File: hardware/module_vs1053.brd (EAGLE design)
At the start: 109.9 x 68.6 mm, 118 parts, among them IC1 IC_USBLC6-2, IC2 LM1117IMPX-3.3, IC3 PIC32MX795F512, IC4 DP83848, IC5 LM1117MPX-2.5, J1 AUDIO_JACK_TRRSSMD_RA, U1 USD-SOCKETUSD, U3 VS1053-L, X2 CRYSTALS-NOGND-CFPX-217, X3 KUSBVX, Y3 CRYSTAL-GROUNDEDSMD-5X3.2

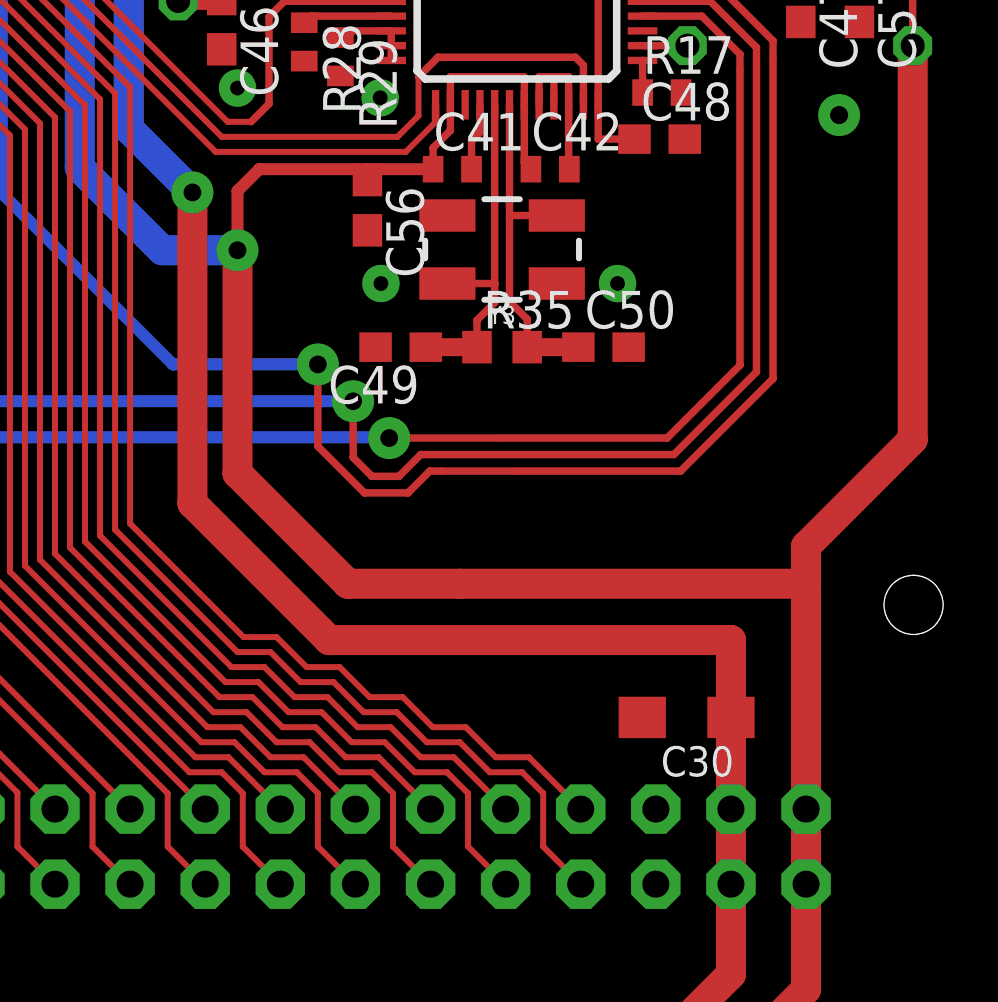
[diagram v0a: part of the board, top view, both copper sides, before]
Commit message: Minor updates in PCB design
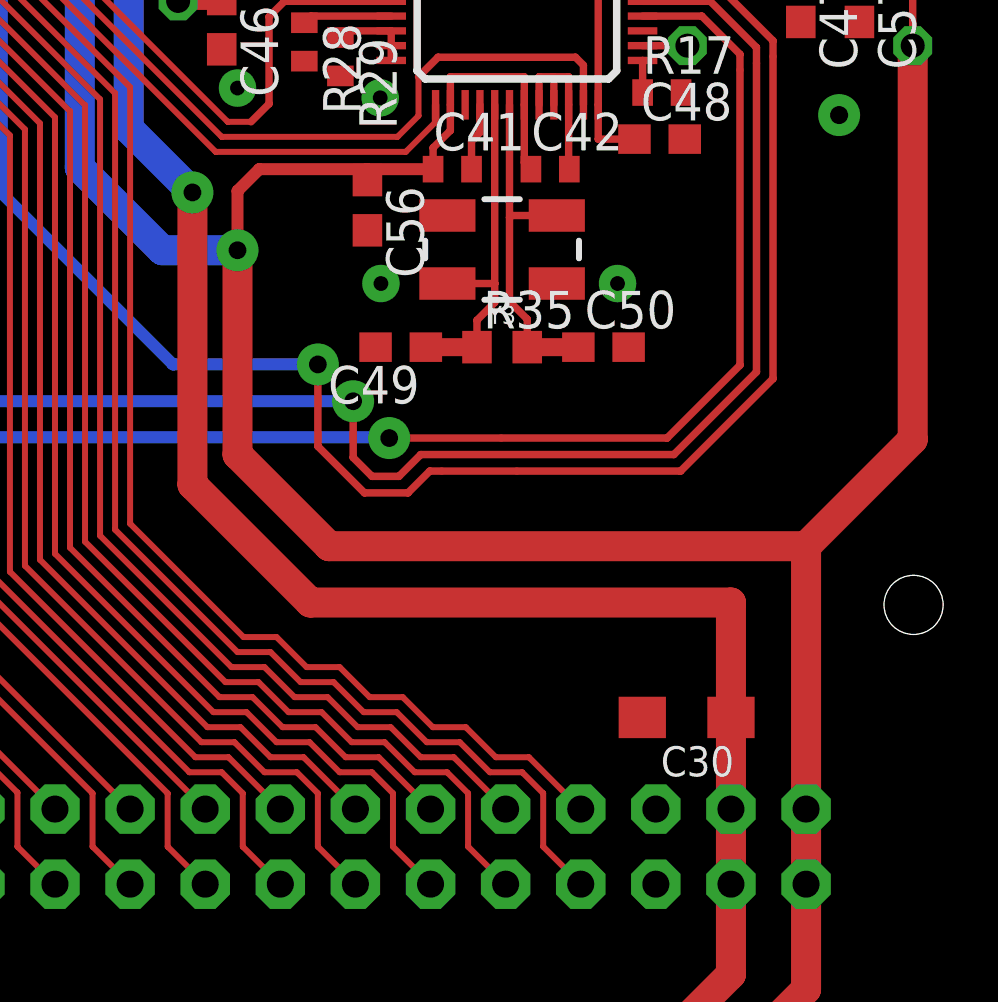
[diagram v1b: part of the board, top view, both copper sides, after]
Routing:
- net 3V: track 525.4 -> 524.4 mm
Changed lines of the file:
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@@
 <contactref element="SV1" pad="34"/>
 <contactref element="SV1" pad="33"/>
-<wire x1="81.9912" y1="23.4188" x2="85.725" y2="19.685" width="1.016" layer="1"/>
-<wire x1="85.725" y1="19.685" x2="89.5096" y2="19.685" width="1.016" layer="1"/>
-<wire x1="89.5096" y1="19.685" x2="100.965" y2="19.685" width="1.016" layer="1"/>
-<wire x1="100.965" y1="19.685" x2="101.219" y2="19.685" width="1.016" layer="1"/>
+<wire x1="81.9912" y1="24.0538" x2="85.09" y2="20.955" width="1.016" layer="1"/>
 <wire x1="98.425" y1="3.175" x2="101.219" y2="5.969" width="1.016" layer="1"/>
-<wire x1="101.219" y1="12.065" x2="101.219" y2="19.431" width="1.016" layer="1"/>
 <wire x1="101.219" y1="9.525" x2="101.219" y2="5.969" width="1.016" layer="1"/>
 <wire x1="101.219" y1="9.525" x2="101.219" y2="12.065" width="1.016" layer="1"/>
 <wire x1="22.8346" y1="10.1828" x2="22.8346" y2="3.175" width="0.6096" layer="1"/>
-<wire x1="89.4588" y1="19.7358" x2="89.5096" y2="19.685" width="0.251459375" layer="1"/>
-<wire x1="81.9912" y1="30.9626" x2="81.9912" y2="23.4188" width="1.016" layer="1"/>
+<wire x1="81.9912" y1="30.9626" x2="81.9912" y2="24.0538" width="1.016" layer="1"/>
 <wire x1="104.8258" y1="37.882" x2="104.8258" y2="40.6146" width="0.251459375" layer="1"/>
 <wire x1="104.8258" y1="37.882" x2="104.8258" y2="24.5618" width="1.016" layer="1"/>
-<wire x1="101.219" y1="19.431" x2="100.965" y2="19.685" width="1.016" layer="1"/>
 <wire x1="99.7338" y1="40.882" x2="100.2538" y2="41.402" width="0.251459375" layer="1"/>
 <wire x1="100.2538" y1="41.402" x2="104.0384" y2="41.402" width="0.251459375" layer="1"/>
@@
 <wire x1="81.9912" y1="30.9626" x2="79.4512" y2="30.9626" width="1.016" layer="16"/>
 <wire x1="79.4512" y1="30.9626" x2="76.6572" y2="33.7566" width="1.016" layer="16"/>
-<wire x1="101.219" y1="19.685" x2="101.219" y2="20.955" width="1.016" layer="1"/>
 <wire x1="101.219" y1="20.955" x2="104.8258" y2="24.5618" width="1.016" layer="1"/>
 <wire x1="84.8106" y1="42.291" x2="81.3562" y2="45.7454" width="0.6096" layer="16"/>
@@
 <wire x1="63.754" y1="59.344" x2="76.6572" y2="46.4408" width="1.016" layer="16"/>
 <wire x1="76.6572" y1="46.4408" x2="76.6572" y2="45.7454" width="1.016" layer="16"/>
+<wire x1="101.219" y1="12.065" x2="101.219" y2="20.955" width="1.016" layer="1"/>
+<wire x1="101.219" y1="20.955" x2="85.09" y2="20.955" width="1.016" layer="1"/>
 </signal>
 <signal name="SOSCI">
@@
 <wire x1="62.9142" y1="54.1542" x2="62.9158" y2="54.1558" width="1.016" layer="1"/>
 <via x="80.4672" y="32.9184" extent="1-16" drill="0.6" diameter="1.4224" shape="octagon"/>
-<wire x1="80.4672" y1="32.9184" x2="80.4672" y2="22.4028" width="1.016" layer="1"/>
+<wire x1="80.4672" y1="32.9184" x2="80.4672" y2="23.0378" width="1.016" layer="1"/>
 <wire x1="78.3082" y1="35.0774" x2="80.4672" y2="32.9184" width="1.016" layer="16"/>
 <contactref element="SV1" pad="32"/>
 <contactref element="SV1" pad="31"/>
-<wire x1="80.4672" y1="22.4028" x2="85.09" y2="17.78" width="1.016" layer="1"/>
-<wire x1="85.09" y1="17.78" x2="98.679" y2="17.78" width="1.016" layer="1"/>
+<wire x1="80.4672" y1="23.0378" x2="84.455" y2="19.05" width="1.016" layer="1"/>
+<wire x1="84.455" y1="19.05" x2="98.679" y2="19.05" width="1.016" layer="1"/>
 <wire x1="98.679" y1="12.065" x2="98.679" y2="15.24" width="1.016" layer="1"/>
-<wire x1="98.679" y1="15.24" x2="98.679" y2="17.78" width="1.016" layer="1"/>
+<wire x1="98.679" y1="15.24" x2="98.679" y2="19.05" width="1.016" layer="1"/>
 <wire x1="98.679" y1="9.525" x2="98.679" y2="12.065" width="1.016" layer="1"/>
 <wire x1="98.679" y1="9.525" x2="98.679" y2="6.477" width="1.016" layer="1"/>

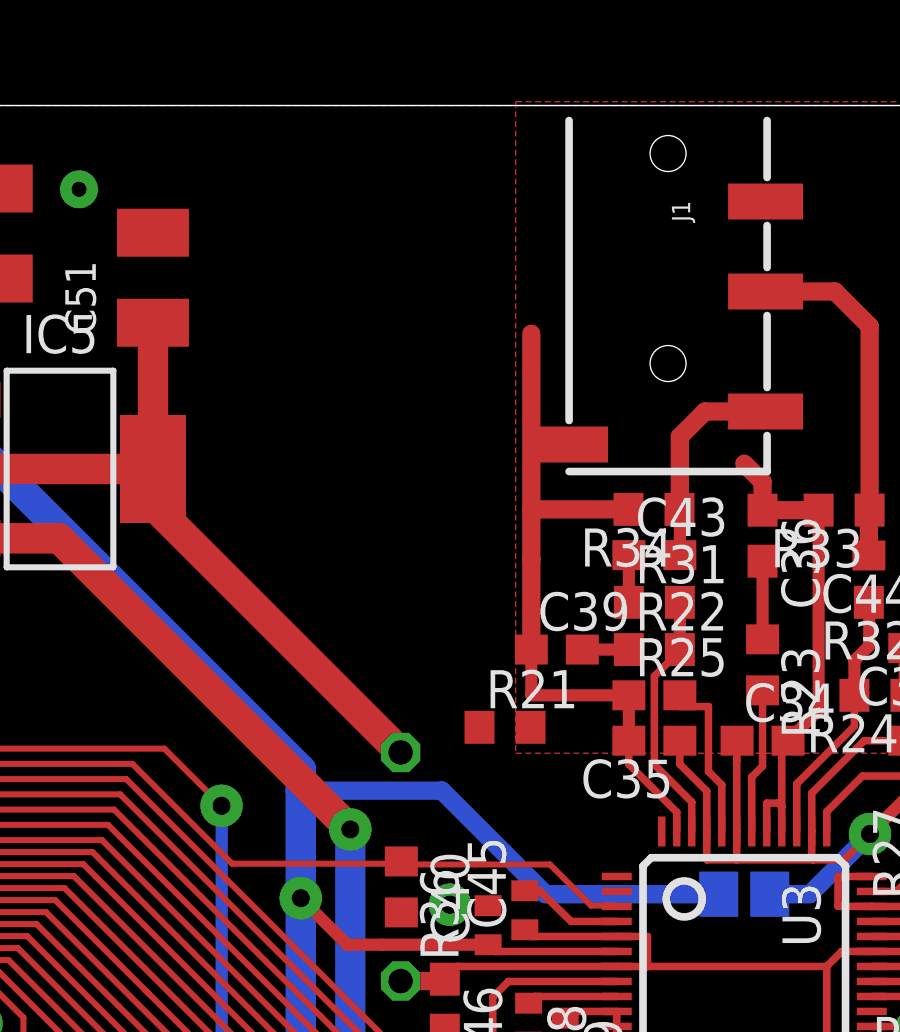
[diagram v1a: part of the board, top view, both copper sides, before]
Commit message: ADC (work in progress)
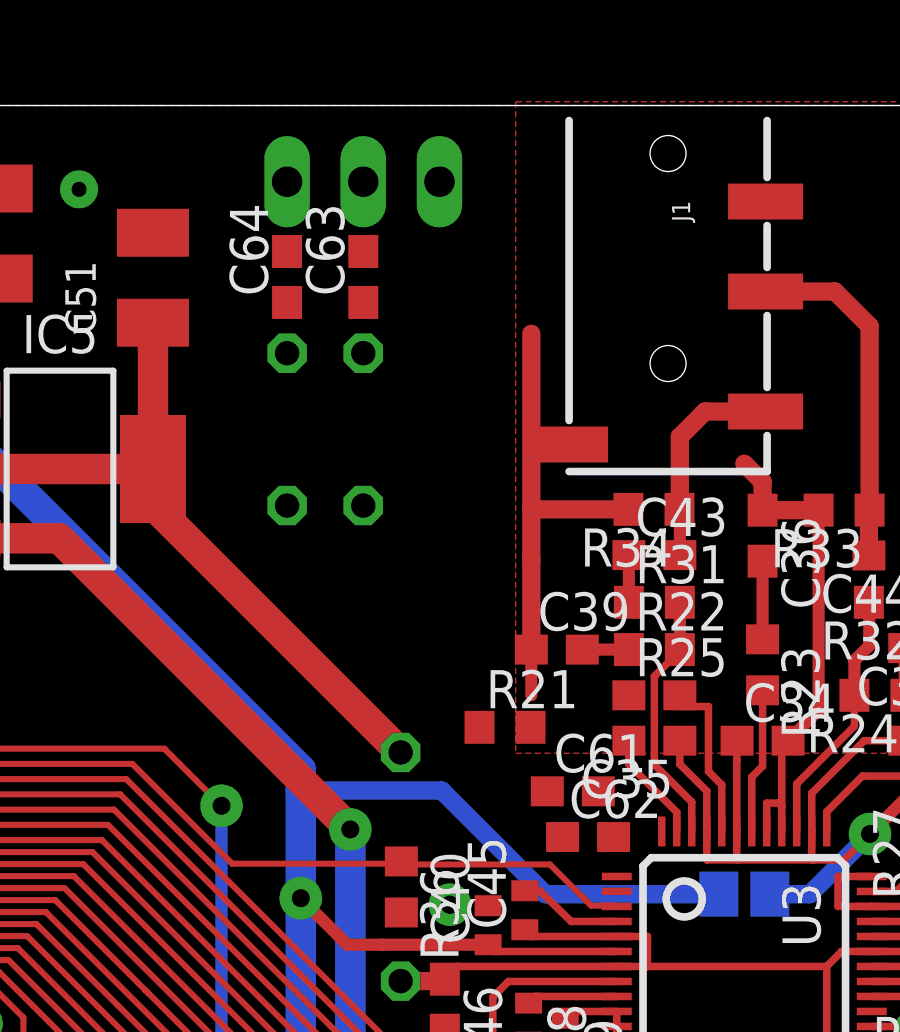
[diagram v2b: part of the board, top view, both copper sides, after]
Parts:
- added C61, C62: 10n, rcl:C0603
- added C63, C64: 1u, rcl:C0603
- added JP1: (no value), pinhead:1X03
- added R12, R37: 470, rcl:0204/5
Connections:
- new net IN_LEFT: C63.2, JP1.2
- new net IN_RIGHT: C64.2, JP1.1
- new net N$13: C62.2, R12.2, U3.1
- new net N$14: C64.1, R37.1
- new net N$15: C63.1, R12.1
- new net N$5: C61.2, R37.2, U3.48
- net VS_AGND: now also C61.1, C62.1, JP1.3
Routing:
- net VS_AGND: track 54.1 -> 49.3 mm
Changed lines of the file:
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@@
 <attribute name="PROD_ID" value="CONN-10676" x="88.9" y="68.58" size="1.778" layer="27" rot="R270" display="off"/>
 </element>
+<element name="C61" library="rcl" package="C0603" value="10n" x="85.725" y="45.72"/>
+<element name="C62" library="rcl" package="C0603" value="10n" x="86.233" y="44.196"/>
+<element name="R12" library="rcl" package="0204/5" value="470" x="78.74" y="57.785" rot="MR270"/>
+<element name="R37" library="rcl" package="0204/5" value="470" x="76.2" y="57.785" rot="MR270"/>
+<element name="C63" library="rcl" package="C0603" value="1u" x="78.74" y="62.865" rot="R90"/>
+<element name="C64" library="rcl" package="C0603" value="1u" x="76.2" y="62.865" rot="R90"/>
+<element name="JP1" library="pinhead" package="1X03" value="" x="78.74" y="66.04" rot="MR180"/>
 </elements>
 <signals>
@@
 <wire x1="92.19" y1="45.327" x2="92.575" y2="45.327" width="0.251459375" layer="1"/>
 <wire x1="92.575" y1="45.327" x2="92.69" y2="45.212" width="0.251459375" layer="1"/>
-<contactref element="R25" pad="1"/>
-<wire x1="87.5928" y1="48.9204" x2="87.5928" y2="47.407" width="0.4064" layer="1"/>
 <contactref element="C36" pad="1"/>
 <contactref element="C39" pad="1"/>
@@
 <wire x1="98.4876" y1="46.5446" x2="98.171" y2="46.228" width="0.251459375" layer="1"/>
 <wire x1="98.171" y1="46.228" x2="95.377" y2="46.228" width="0.251459375" layer="1"/>
-<wire x1="87.5928" y1="48.9204" x2="84.3416" y2="48.9204" width="0.4064" layer="1"/>
 <wire x1="84.3416" y1="50.4444" x2="84.3416" y2="53.467" width="0.6096" layer="1"/>
 <contactref element="R34" pad="2"/>
@@
 <contactref element="U3" pad="47"/>
 <contactref element="J1" pad="EARTH"/>
+<contactref element="JP1" pad="3"/>
+<contactref element="C61" pad="1"/>
+<contactref element="R25" pad="1"/>
+<contactref element="C62" pad="1"/>
+<wire x1="84.3416" y1="60.9736" x2="81.28" y2="66.04" width="0" layer="19" extent="1-1"/>
+<wire x1="84.875" y1="45.72" x2="84.3144" y2="47.8536" width="0" layer="19" extent="1-1"/>
+<wire x1="85.383" y1="44.196" x2="84.875" y2="45.72" width="0" layer="19" extent="1-1"/>
 </signal>
 <signal name="VS_CVDD">
@@
 <wire x1="58.7756" y1="7.7216" x2="60.579" y2="9.525" width="0.2032" layer="1"/>
 </signal>
+<signal name="N$5">
+<contactref element="C61" pad="2"/>
+<contactref element="R37" pad="2"/>
+<contactref element="U3" pad="48"/>
+<wire x1="88.69" y1="44.382" x2="86.575" y2="45.72" width="0" layer="19" extent="1-1"/>
+<wire x1="76.2" y1="55.245" x2="86.575" y2="45.72" width="0" layer="19" extent="1-1"/>
+</signal>
+<signal name="N$13">
+<contactref element="C62" pad="2"/>
+<contactref element="R12" pad="2"/>
+<contactref element="U3" pad="1"/>
+<wire x1="87.083" y1="44.196" x2="78.74" y2="55.245" width="0" layer="19" extent="1-1"/>
+<wire x1="87.19" y1="42.882" x2="87.083" y2="44.196" width="0" layer="19" extent="1-1"/>
+</signal>
+<signal name="N$14">
+<contactref element="R37" pad="1"/>
+<contactref element="C64" pad="1"/>
+<wire x1="76.2" y1="60.325" x2="76.2" y2="62.015" width="0" layer="19" extent="1-1"/>
+</signal>
+<signal name="N$15">
+<contactref element="R12" pad="1"/>
+<contactref element="C63" pad="1"/>
+<wire x1="78.74" y1="60.325" x2="78.74" y2="62.015" width="0" layer="19" extent="1-1"/>
+</signal>
+<signal name="IN_LEFT">
+<contactref element="JP1" pad="2"/>
+<contactref element="C63" pad="2"/>
+<wire x1="78.74" y1="63.715" x2="78.74" y2="66.04" width="0" layer="19" extent="1-1"/>
+</signal>
+<signal name="IN_RIGHT">
+<contactref element="C64" pad="2"/>
+<contactref element="JP1" pad="1"/>
+<wire x1="76.2" y1="63.715" x2="76.2" y2="66.04" width="0" layer="19" extent="1-1"/>
+</signal>
 </signals>
